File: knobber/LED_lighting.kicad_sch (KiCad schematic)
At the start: 34 parts, among them U201 SN74LV1T34DBV

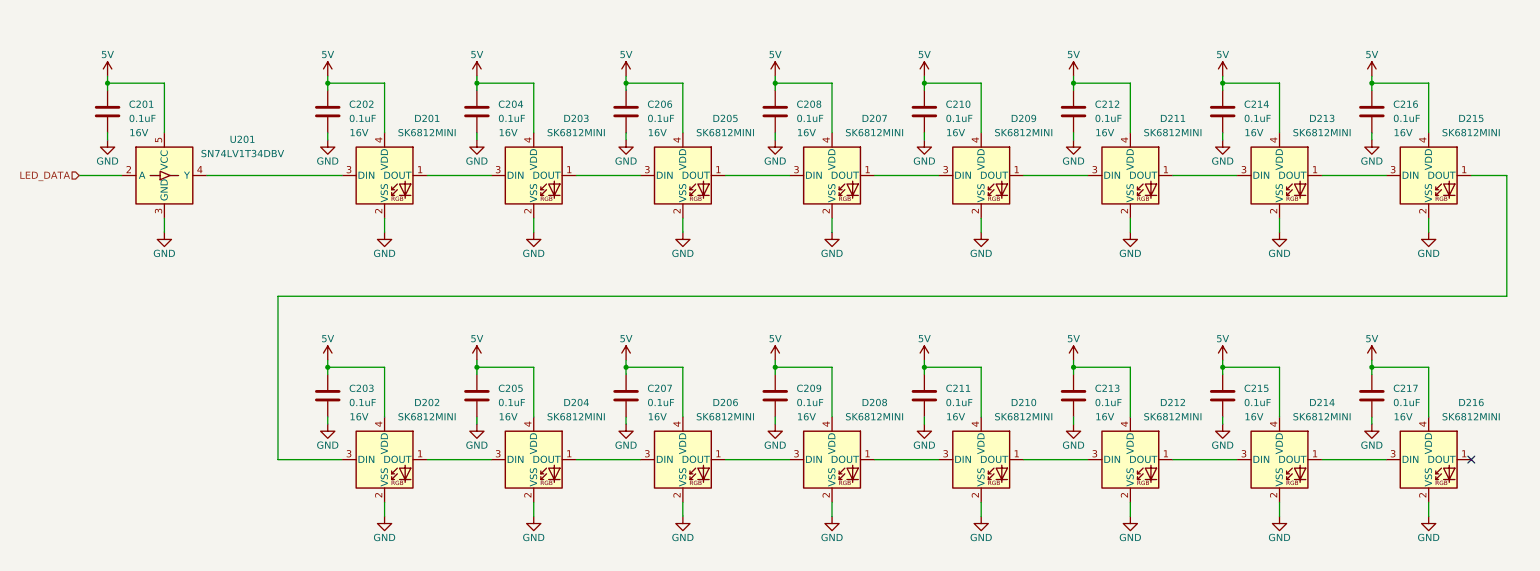
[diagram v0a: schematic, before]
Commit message: Updated schematic & PCB
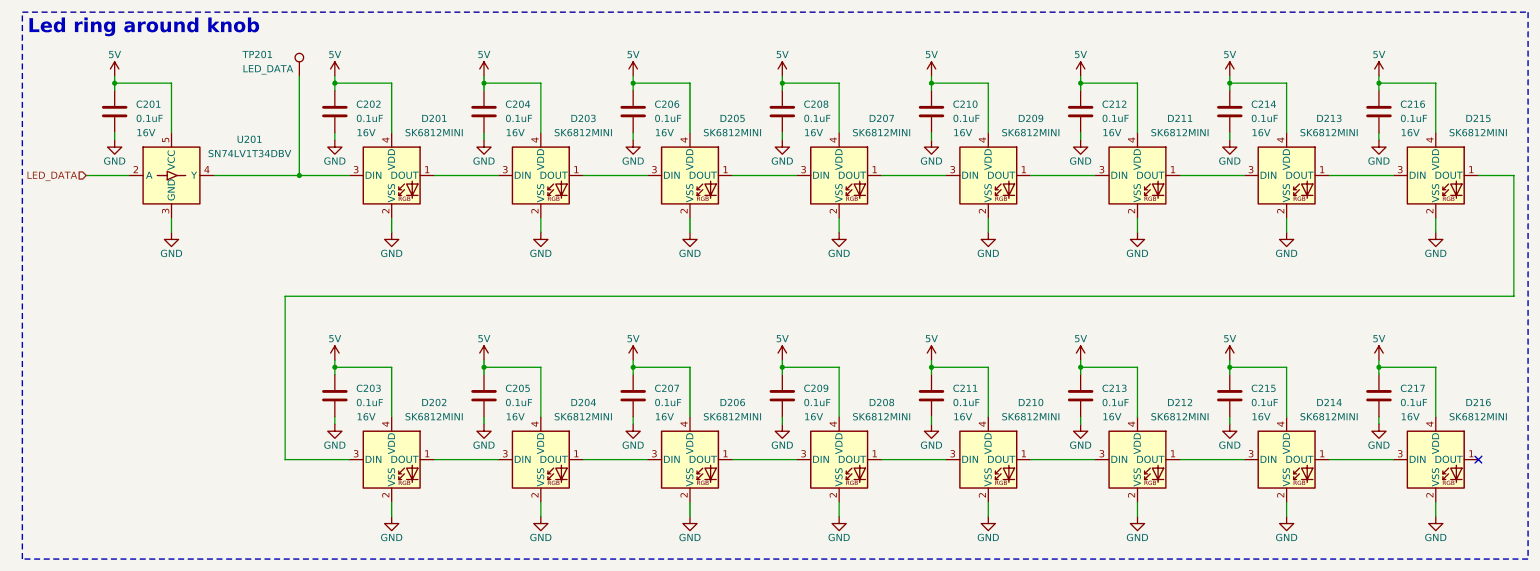
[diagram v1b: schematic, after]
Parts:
- added TP201: LED_DATA, TestPoint:TestPoint_Pad_D1.0mm, symbol Connector:TestPoint
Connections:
- net at D201.3 (DIN), U201.4 (Y): now also TP201.1
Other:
- moved on the sheet: C201, C202, C203, C204, C205, C206, C207, C208, C209, C210, C211, C212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
